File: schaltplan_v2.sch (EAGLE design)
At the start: 18 parts

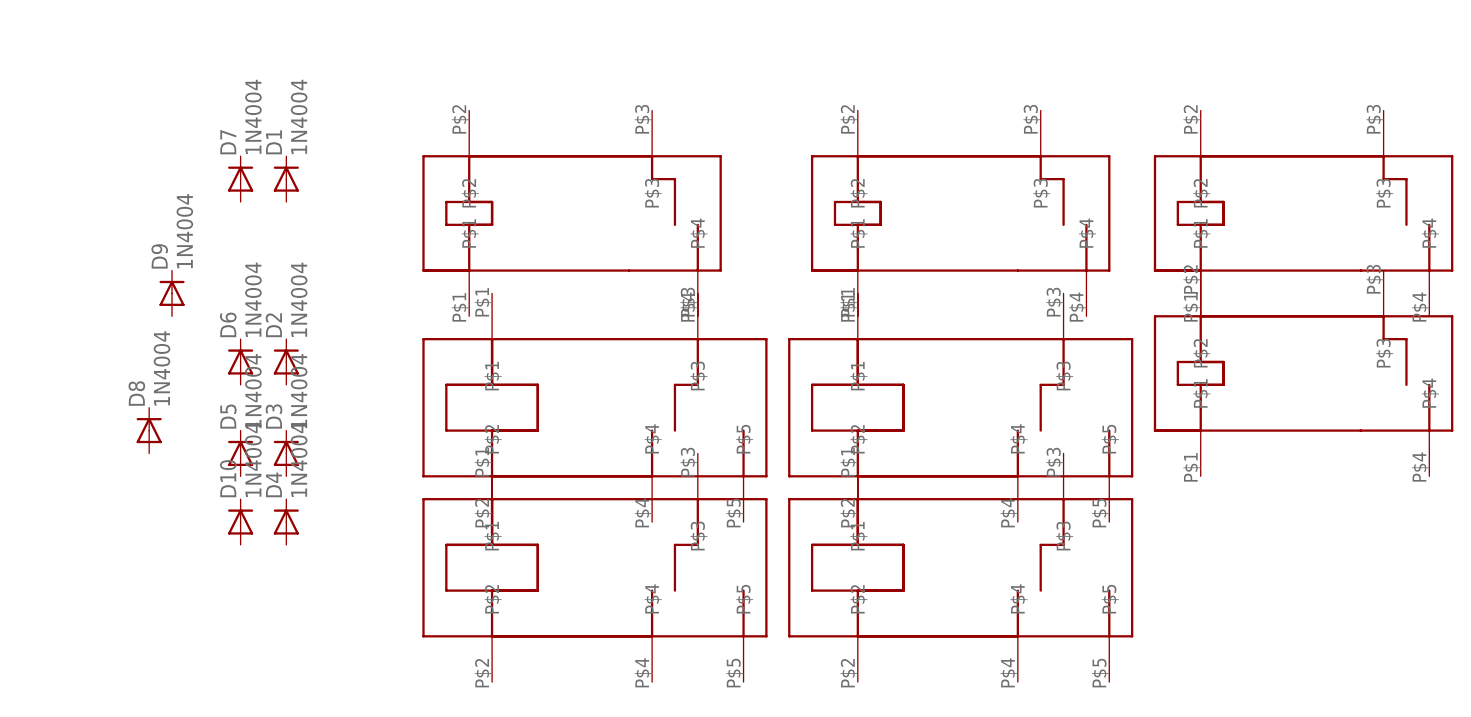
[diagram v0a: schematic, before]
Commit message: layout/board redesign
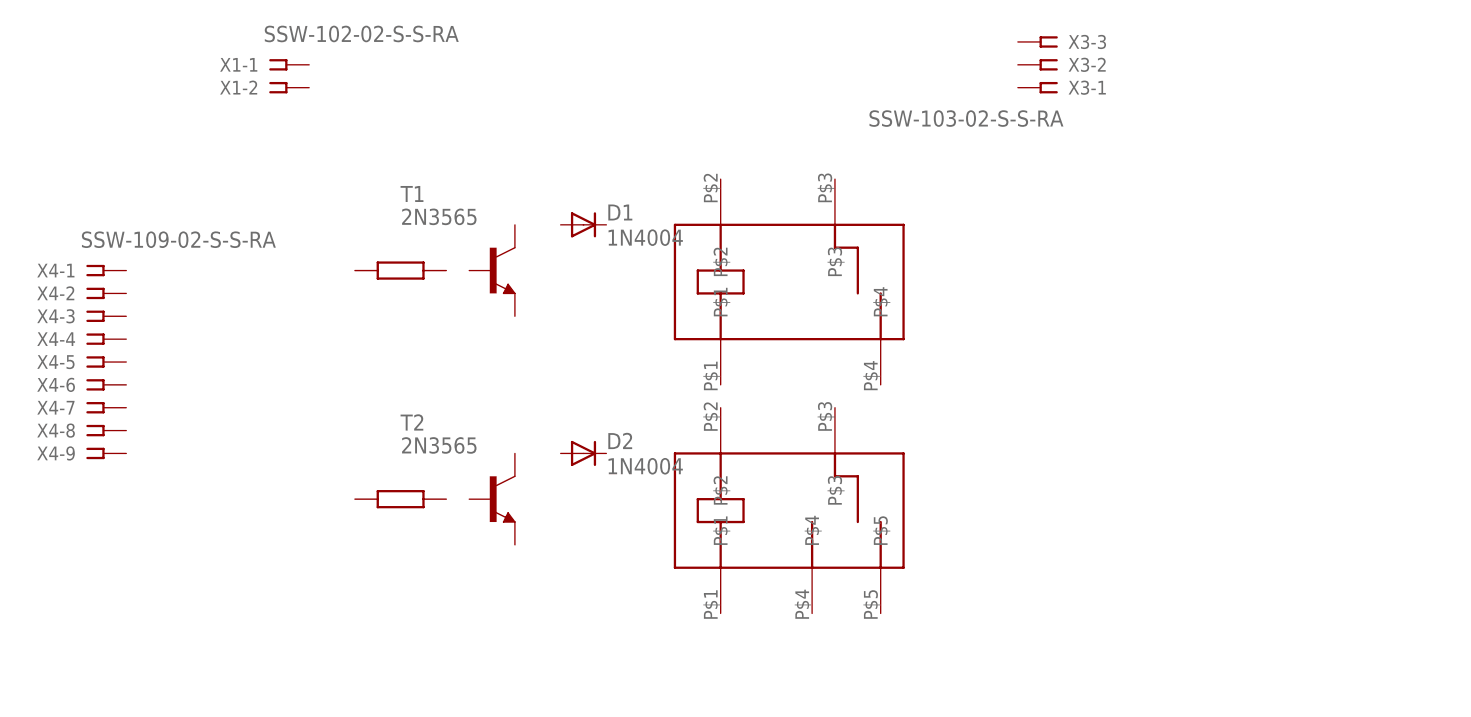
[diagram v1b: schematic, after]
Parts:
- removed D10, D3, D4, D5, D6, D7, D8, D9: 1N4004, diode:1N4004
- removed U$3, U$4, U$5: JS_05_MN_KT, n39:JS_05_MN_KT
- removed U$6, U$7, U$8: JS_05_N_K, n39:JS_05_N_K
- added T1, T2: 2N3565, transistor:2N3565
- added X1: SSW-102-02-S-S-RA, con-samtec:SSW-102-02-S-S-RA
- added X3: SSW-103-02-S-S-RA, con-samtec:SSW-103-02-S-S-RA
- added X4: SSW-109-02-S-S-RA, con-samtec:SSW-109-02-S-S-RA
- U$1: value JS_05_N_K -> JS_05_MN_KT; device n39:JS_05_N_K -> n39:JS_05_MN_KT
- U$2: value JS_05_MN_KT -> JS_05_N_K; device n39:JS_05_MN_KT -> n39:JS_05_N_K
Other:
- moved on the sheet: D1, D2
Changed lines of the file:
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@@
 <parts>
 <part name="D1" library="diode" deviceset="1N4004" device=""/>
+<part name="U$1" library="n39" deviceset="JS_05_MN_KT" device=""/>
+<part name="U$2" library="n39" deviceset="JS_05_N_K" device=""/>
+<part name="T1" library="transistor" deviceset="2N3565" device=""/>
+<part name="R1" library="docu-dummy" deviceset="R" device=""/>
 <part name="D2" library="diode" deviceset="1N4004" device=""/>
-<part name="U$1" library="n39" deviceset="JS_05_N_K" device=""/>
-<part name="U$2" library="n39" deviceset="JS_05_MN_KT" device=""/>
-<part name="U$3" library="n39" deviceset="JS_05_MN_KT" device=""/>
-<part name="U$4" library="n39" deviceset="JS_05_MN_KT" device=""/>
-<part name="U$5" library="n39" deviceset="JS_05_MN_KT" device=""/>
-<part name="U$6" library="n39" deviceset="JS_05_N_K" device=""/>
-<part name="U$7" library="n39" deviceset="JS_05_N_K" device=""/>
-<part name="U$8" library="n39" deviceset="JS_05_N_K" device=""/>
-<part name="D3" library="diode" deviceset="1N4004" device=""/>
-<part name="D4" library="diode" deviceset="1N4004" device=""/>
-<part name="D5" library="diode" deviceset="1N4004" device=""/>
-<part name="D6" library="diode" deviceset="1N4004" device=""/>
-<part name="D7" library="diode" deviceset="1N4004" device=""/>
-<part name="D8" library="diode" deviceset="1N4004" device=""/>
-<part name="D9" library="diode" deviceset="1N4004" device=""/>
-<part name="D10" library="diode" deviceset="1N4004" device=""/>
+<part name="T2" library="transistor" deviceset="2N3565" device=""/>
+<part name="R2" library="docu-dummy" deviceset="R" device=""/>
+<part name="X1" library="con-samtec" deviceset="SSW-102-02-S-S" device="-RA"/>
+<part name="X3" library="con-samtec" deviceset="SSW-103-02-S-S" device="-RA"/>
+<part name="X4" library="con-samtec" deviceset="SSW-109-02-S-S" device="-RA"/>
 </parts>
 <sheets>
@@
 </plain>
 <instances>
-<instance part="D1" gate="1" x="38.1" y="58.42" rot="R90"/>
-<instance part="D2" gate="1" x="38.1" y="38.1" rot="R90"/>
-<instance part="U$1" gate="G$1" x="96.52" y="20.32"/>
-<instance part="U$2" gate="G$1" x="53.34" y="48.26"/>
-<instance part="U$3" gate="G$1" x="96.52" y="48.26"/>
-<instance part="U$4" gate="G$1" x="134.62" y="48.26"/>
-<instance part="U$5" gate="G$1" x="134.62" y="30.48"/>
-<instance part="U$6" gate="G$1" x="96.52" y="2.54"/>
-<instance part="U$7" gate="G$1" x="137.16" y="20.32"/>
-<instance part="U$8" gate="G$1" x="137.16" y="2.54"/>
-<instance part="D3" gate="1" x="38.1" y="27.94" rot="R90"/>
-<instance part="D4" gate="1" x="38.1" y="20.32" rot="R90"/>
-<instance part="D5" gate="1" x="33.02" y="27.94" rot="R90"/>
-<instance part="D6" gate="1" x="33.02" y="38.1" rot="R90"/>
-<instance part="D7" gate="1" x="33.02" y="58.42" rot="R90"/>
-<instance part="D8" gate="1" x="22.86" y="30.48" rot="R90"/>
-<instance part="D9" gate="1" x="25.4" y="45.72" rot="R90"/>
-<instance part="D10" gate="1" x="33.02" y="20.32" rot="R90"/>
+<instance part="D1" gate="1" x="71.12" y="53.34"/>
+<instance part="U$1" gate="G$1" x="93.98" y="45.72"/>
+<instance part="U$2" gate="G$1" x="93.98" y="20.32"/>
+<instance part="T1" gate="G$1" x="60.96" y="48.26"/>
+<instance part="R1" gate="G$1" x="50.8" y="48.26"/>
+<instance part="D2" gate="1" x="71.12" y="27.94"/>
+<instance part="T2" gate="G$1" x="60.96" y="22.86"/>
+<instance part="R2" gate="G$1" x="50.8" y="22.86"/>
+<instance part="X1" gate="-1" x="38.1" y="71.12"/>
+<instance part="X1" gate="-2" x="38.1" y="68.58"/>
+<instance part="X3" gate="-1" x="121.92" y="68.58" rot="R180"/>
+<instance part="X3" gate="-2" x="121.92" y="71.12" rot="R180"/>
+<instance part="X3" gate="-3" x="121.92" y="73.66" rot="R180"/>
+<instance part="X4" gate="-1" x="17.78" y="48.26"/>
+<instance part="X4" gate="-2" x="17.78" y="45.72"/>
+<instance part="X4" gate="-3" x="17.78" y="43.18"/>
+<instance part="X4" gate="-4" x="17.78" y="40.64"/>
+<instance part="X4" gate="-5" x="17.78" y="38.1"/>
+<instance part="X4" gate="-6" x="17.78" y="35.56"/>
+<instance part="X4" gate="-7" x="17.78" y="33.02"/>
+<instance part="X4" gate="-8" x="17.78" y="30.48"/>
+<instance part="X4" gate="-9" x="17.78" y="27.94"/>
 </instances>
 <busses>

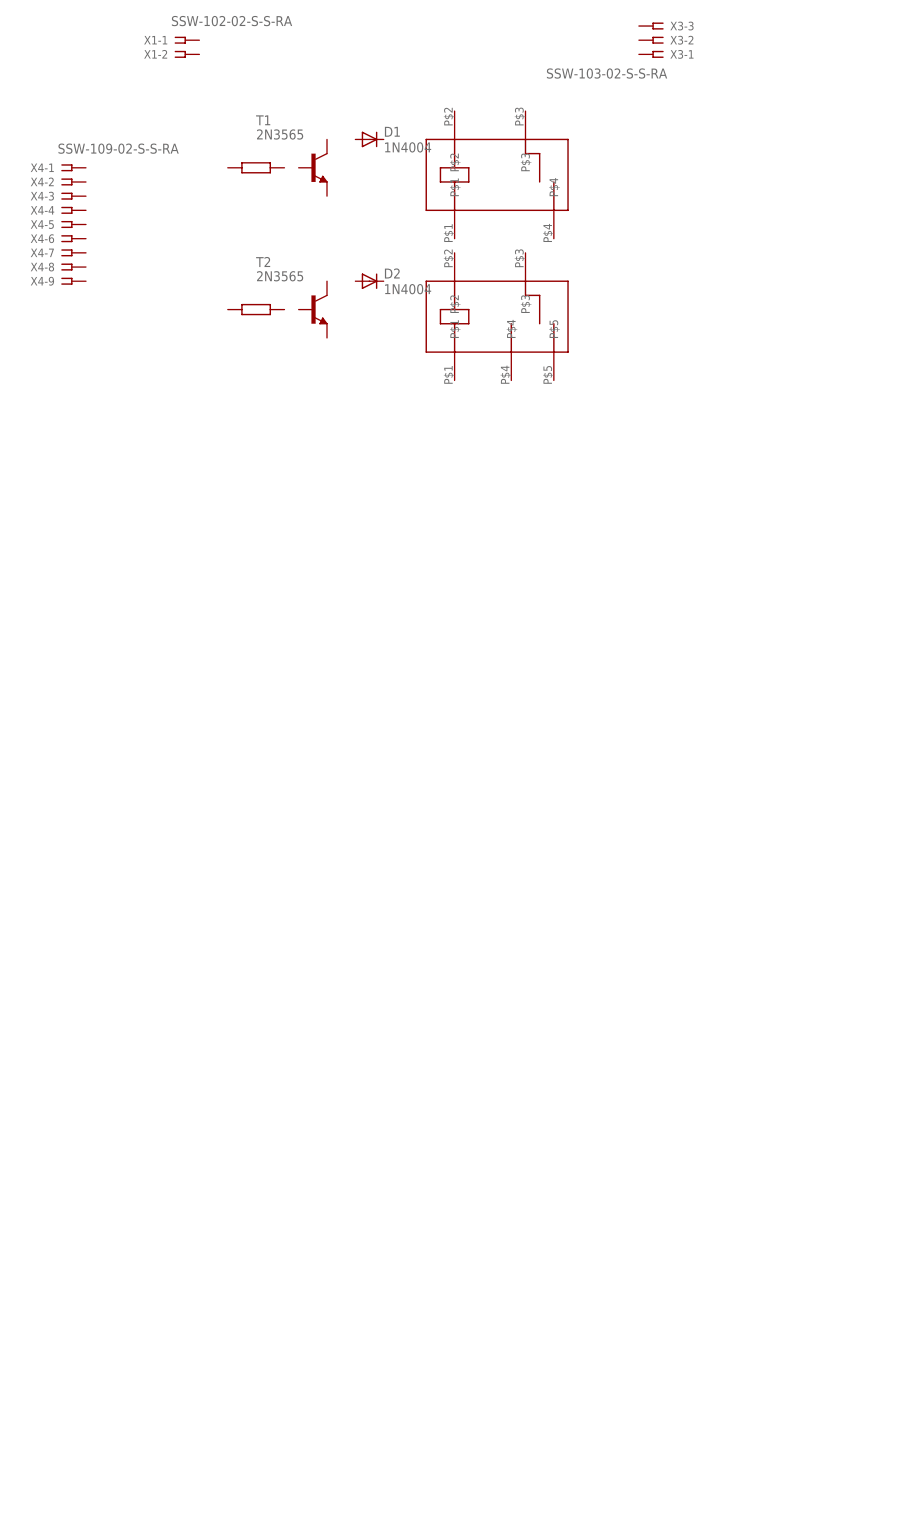
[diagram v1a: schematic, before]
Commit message: schaltplan_v2 finalized
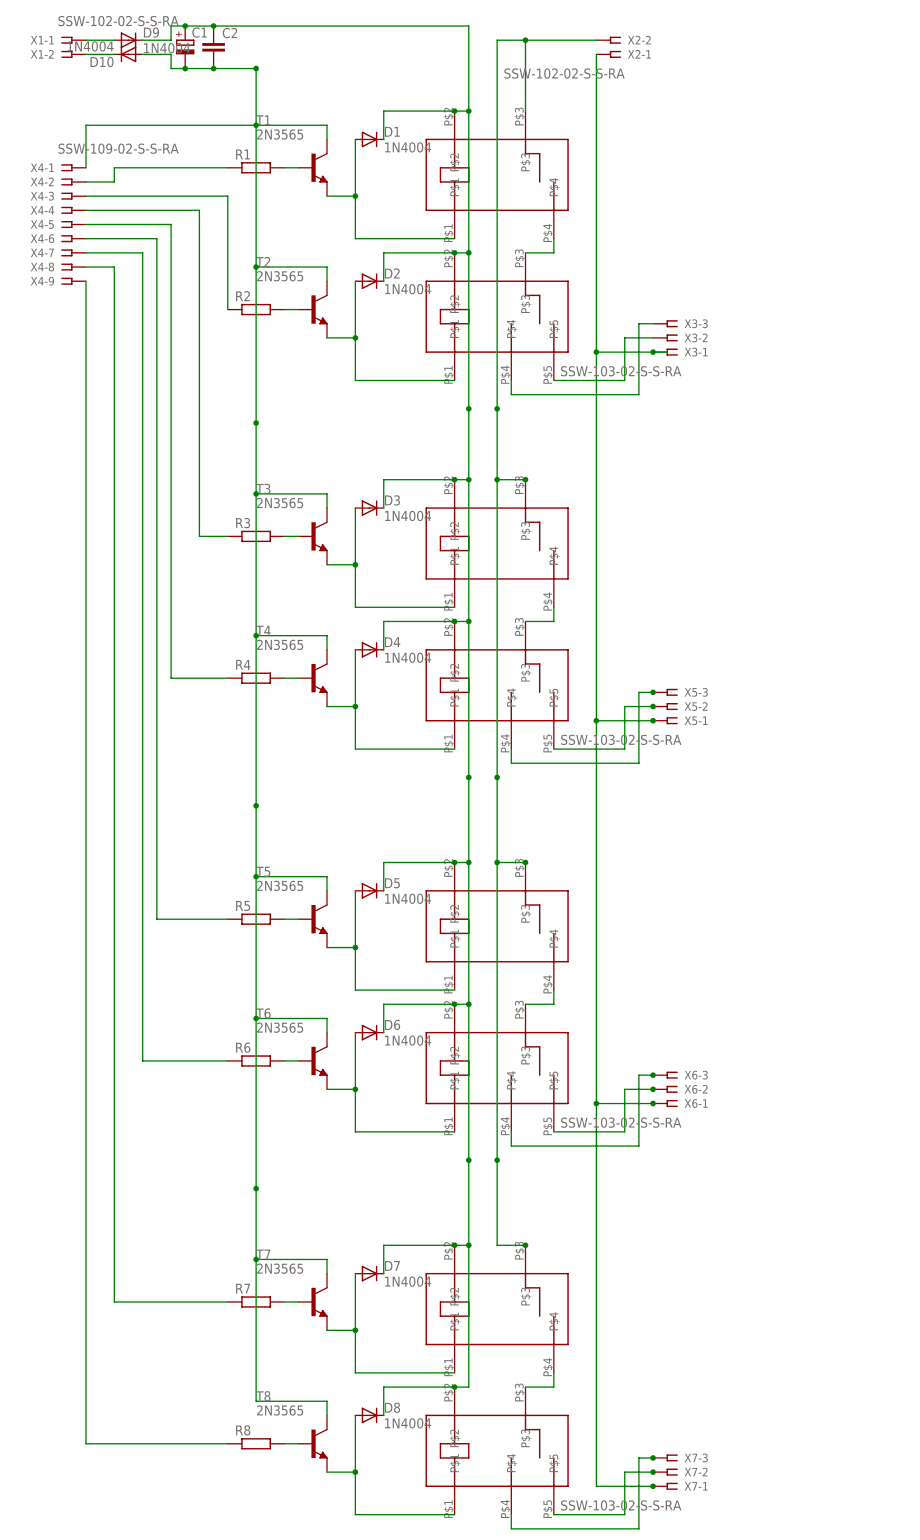
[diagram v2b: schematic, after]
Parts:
- added C1: (no value), rcl:CPOL-EUE3.5-8
- added C2: (no value), rcl:C-EU025-030X050
- added D10, D3, D4, D5, D6, D7, D8, D9: 1N4004, diode:1N4004
- added R1, R2, R3, R4, R5, R6, R7, R8: (no value), resistor:R-EU_0204/2V
- added T3, T4, T5, T6, T7, T8: 2N3565, transistor:2N3565
- added U$3, U$5, U$7: JS_05_MN_KT, n39:JS_05_MN_KT
- added U$4, U$6, U$8: JS_05_N_K, n39:JS_05_N_K
- added X2: SSW-102-02-S-S-RA, con-samtec:SSW-102-02-S-S-RA
- added X5, X6, X7: SSW-103-02-S-S-RA, con-samtec:SSW-103-02-S-S-RA
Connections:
- new net N$1: X2-1.1, X3-1.1, X5-1.1, X6-1.1, X7-1.1
- new net N$10: C1.-, C2.2, D10.A, T1.C, T2.C, T3.C, T4.C, T5.C, T6.C, T7.C, T8.C, X4-1.1
- new net N$11: R2.1, X4-3.1
- new net N$12: D2.A, T2.E, U$2.P$1
- new net N$13: R6.2, T6.B
- new net N$14: R3.1, X4-4.1
- new net N$16: U$4.P$5, X5-2.1
- new net N$17: U$4.P$4, X5-3.1
- new net N$18: U$3.P$4, U$4.P$3
- new net N$2: U$2.P$5, X3-2.1
- new net N$20: D3.A, T3.E, U$3.P$1
- new net N$21: C1.+, C2.1, D1.C, D2.C, D3.C, D4.C, D5.C, D6.C, D7.C, D8.C, D9.C, U$1.P$2, U$2.P$2, U$3.P$2, U$4.P$2, U$5.P$2, U$6.P$2, U$7.P$2, U$8.P$2
- new net N$22: R3.2, T3.B
- new net N$23: R4.1, X4-5.1
- new net N$25: D4.A, T4.E, U$4.P$1
- new net N$26: R5.1, X4-6.1
- new net N$27: R2.2, T2.B
- new net N$28: R4.2, T4.B
- new net N$3: U$2.P$4, X3-3.1
- new net N$30: U$6.P$5, X6-2.1
- new net N$31: U$6.P$4, X6-3.1
- new net N$32: U$5.P$4, U$6.P$3
- new net N$34: D5.A, T5.E, U$5.P$1
- new net N$36: R5.2, T5.B
- new net N$37: R6.1, X4-7.1
- new net N$39: D6.A, T6.E, U$6.P$1
- new net N$4: U$1.P$4, U$2.P$3
- new net N$40: R8.2, T8.B
- new net N$42: U$8.P$5, X7-2.1
- new net N$43: U$8.P$4, X7-3.1
- new net N$44: U$7.P$4, U$8.P$3
- new net N$46: D7.A, T7.E, U$7.P$1
- new net N$48: R7.2, T7.B
- new net N$49: R7.1, X4-8.1
- new net N$5: U$1.P$3, U$3.P$3, U$5.P$3, U$7.P$3, X2-2.1
- new net N$51: D8.A, T8.E, U$8.P$1
- new net N$53: D9.A, X1-1.1
- new net N$54: D10.C, X1-2.1
- new net N$6: D1.A, T1.E, U$1.P$1
- new net N$7: R8.1, X4-9.1
- new net N$8: R1.2, T1.B
- new net N$9: R1.1, X4-2.1
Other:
- moved on the sheet: X1-1, X1-2, X3-1, X3-2, X3-3

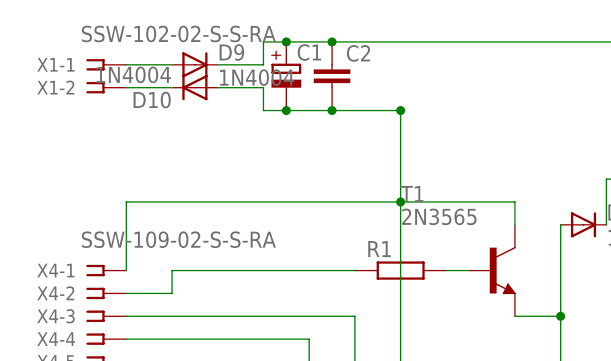
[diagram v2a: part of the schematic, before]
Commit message: more fixes
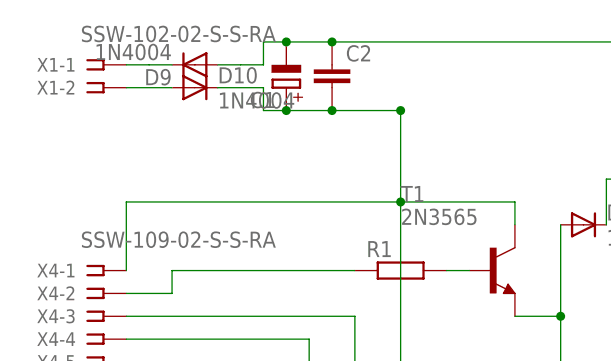
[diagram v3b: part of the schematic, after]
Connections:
- removed net N$10: C1.-, C2.2, D10.A, T1.C, T2.C, T3.C, T4.C, T5.C, T6.C, T7.C, T8.C, X4-1.1
- removed net N$21: C1.+, C2.1, D1.C, D2.C, D3.C, D4.C, D5.C, D6.C, D7.C, D8.C, D9.C, U$1.P$2, U$2.P$2, U$3.P$2, U$4.P$2, U$5.P$2, U$6.P$2, U$7.P$2, U$8.P$2
- removed net N$53: D9.A, X1-1.1
- removed net N$54: D10.C, X1-2.1
- new net N$15: D9.C, X1-1.1
- new net N$19: D10.A, X1-2.1
- new net N$24: C1.+, C2.2, D10.C, T1.C, T2.C, T3.C, T4.C, T5.C, T6.C, T7.C, T8.C, X4-1.1
- new net N$29: C1.-, C2.1, D1.C, D2.C, D3.C, D4.C, D5.C, D6.C, D7.C, D8.C, D9.A, U$1.P$2, U$2.P$2, U$3.P$2, U$4.P$2, U$5.P$2, U$6.P$2, U$7.P$2, U$8.P$2
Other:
- moved on the sheet: C1, D10, D9
